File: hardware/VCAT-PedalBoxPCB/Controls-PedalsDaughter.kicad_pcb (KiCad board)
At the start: 2 copper layers, 53 x 58.6 mm, 36 parts, among them J1 MX150_02x03_Vertical, J6 MX150_02x10_Vertical, J7 53307-2471, U3 TLV9301xDCK, U4 TLV70130DBVR, U5 AMC1300BDWV, U6 TLV9301xDCK

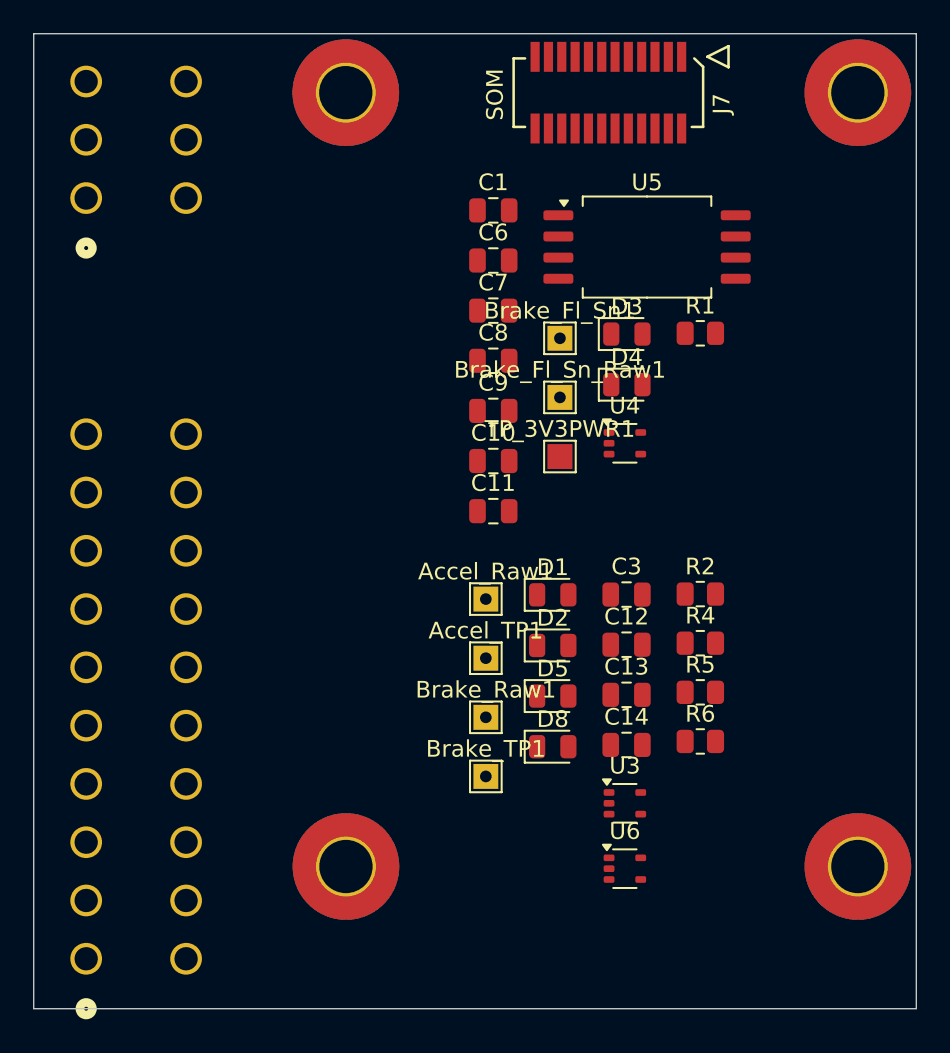
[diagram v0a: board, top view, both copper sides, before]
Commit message: pcb design review #1
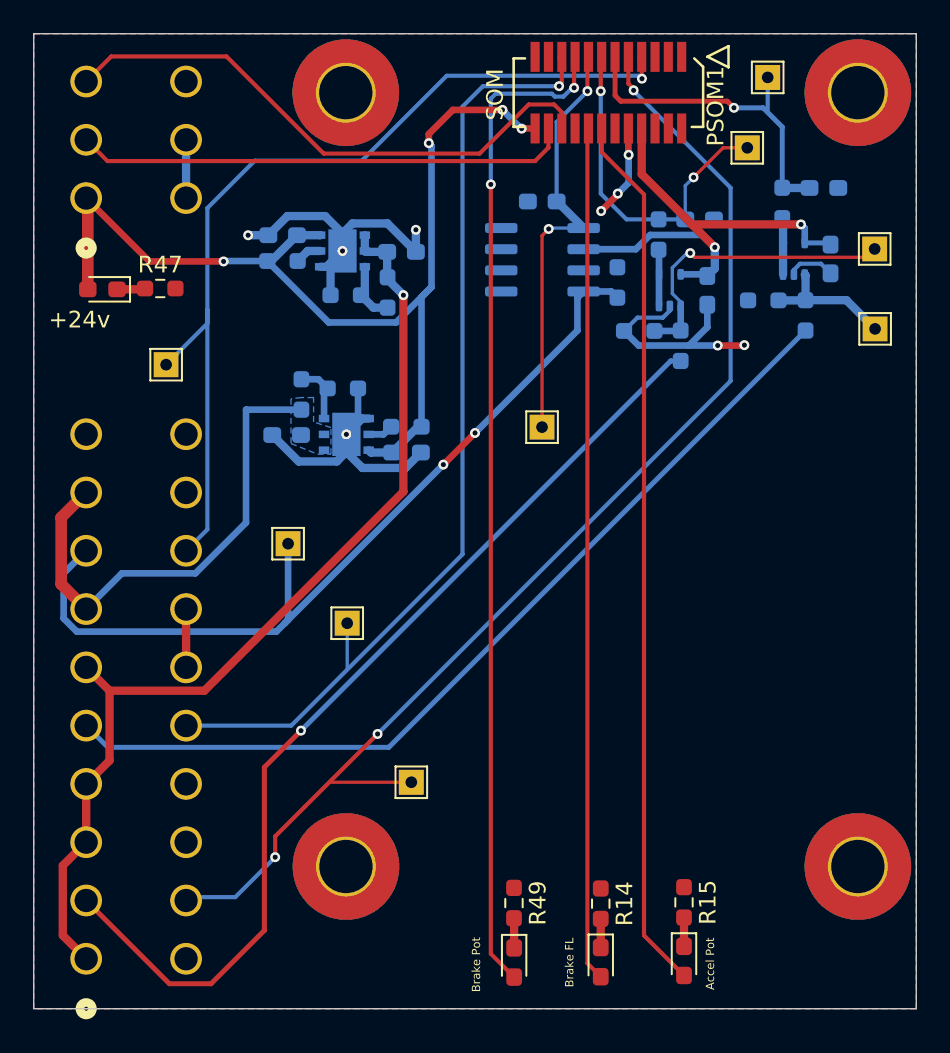
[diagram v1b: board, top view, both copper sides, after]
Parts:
- removed Accel_Raw1: Accel_Raw_TP, TestPoint:TestPoint_THTPad_1.5x1.5mm_Drill0.7mm
- removed Accel_TP1: Accel, TestPoint:TestPoint_THTPad_1.5x1.5mm_Drill0.7mm
- removed Brake_Fl_Sn1: Brake_Fl_Sn_TP, TestPoint:TestPoint_THTPad_1.5x1.5mm_Drill0.7mm
- removed Brake_Fl_Sn_Raw1: Brake_Fl_Sn_Raw_TP, TestPoint:TestPoint_THTPad_1.5x1.5mm_Drill0.7mm
- removed Brake_Raw1: Brake_Raw_TP, TestPoint:TestPoint_THTPad_1.5x1.5mm_Drill0.7mm
- removed Brake_TP1: Brake, TestPoint:TestPoint_THTPad_1.5x1.5mm_Drill0.7mm
- removed C10: 1uF, Capacitor_SMD:C_0805_2012Metric
- removed C11: 100uF, Capacitor_SMD:C_0805_2012Metric
- removed C12, C14: 1nf, Capacitor_SMD:C_0805_2012Metric
- removed C13: 0.1uf, Capacitor_SMD:C_0805_2012Metric
- removed D1, D2, D3, D4, D5, D8: MBR, Diode_SMD:D_0805_2012Metric
- removed TP_3V3PWR1: +3V3PWR, TestPoint:TestPoint_Pad_1.5x1.5mm
- removed U5: AMC1300BDWV, Package_SO:SOIC-8_7.5x5.85mm_P1.27mm
- added +24v: PedalsBoard_Status_Red, LED_SMD:LED_0603_1608Metric_Pad1.05x0.95mm_HandSolder, F.Cu at (125.1, 86.1)
- added Accel Pot: 0603_SMD, LED_SMD:LED_0603_1608Metric_Pad1.05x0.95mm_HandSolder, F.Cu at (160.0, 126.4)
- added AccelPot_Raw: Raw_TP, TestPoint:TestPoint_THTPad_1.5x1.5mm_Drill0.7mm, F.Cu at (171.5, 88.5)
- added AccelPot_Redundant: AccelPotSig, TestPoint:TestPoint_THTPad_1.5x1.5mm_Drill0.7mm, F.Cu at (139.8, 106.2)
- added Accel_GPIO: Accel, TestPoint:TestPoint_THTPad_1.5x1.5mm_Drill0.7mm, F.Cu at (165.0, 73.4)
- added Brake FL: 0603_SMD, LED_SMD:LED_0603_1608Metric_Pad1.05x0.95mm_HandSolder, F.Cu at (155.0, 126.5)
- added Brake Pot: 0603_SMD, LED_SMD:LED_0603_1608Metric_Pad1.05x0.95mm_HandSolder, F.Cu at (149.8, 126.5)
- added BrakeFL_Raw: Brake_Fl_Sn_Raw_TP, TestPoint:TestPoint_THTPad_1.5x1.5mm_Drill0.7mm, F.Cu at (136.2, 101.4)
- added BrakeFl_GPIO: Brake_Fl_Sn_TP, TestPoint:TestPoint_THTPad_1.5x1.5mm_Drill0.7mm, F.Cu at (151.5, 94.4)
- added BrakePot_GPIO: Accel, TestPoint:TestPoint_THTPad_1.5x1.5mm_Drill0.7mm, F.Cu at (163.8, 77.6)
- added BrakePot_Raw: Raw_TP, TestPoint:TestPoint_THTPad_1.5x1.5mm_Drill0.7mm, F.Cu at (171.4, 83.7)
- added BrakePot_Redundant: BrakePotSig, TestPoint:TestPoint_THTPad_1.5x1.5mm_Drill0.7mm, F.Cu at (143.6, 115.7)
- added BrakePress_Redundant: BrakePressSig, TestPoint:TestPoint_THTPad_1.5x1.5mm_Drill0.7mm, F.Cu at (128.9, 90.6)
- added C2: 0.1uf, Capacitor_SMD:C_0603_1608Metric_Pad1.08x0.95mm_HandSolder, B.Cu at (161.4, 86.2)
- added C4: 1uF, Capacitor_SMD:C_0603_1608Metric_Pad1.08x0.95mm_HandSolder, B.Cu at (143.0, 83.8)
- added C5: 1uF, Capacitor_SMD:C_0603_1608Metric_Pad1.08x0.95mm_HandSolder, B.Cu at (135.9, 82.8)
- added R10: 1k, Resistor_SMD:R_0603_1608Metric_Pad0.98x0.95mm_HandSolder, B.Cu at (135.9, 84.4)
- added R11: 100, Resistor_SMD:R_0603_1608Metric_Pad0.98x0.95mm_HandSolder, B.Cu at (165.9, 80.9)
- added R12: 100, Resistor_SMD:R_0603_1608Metric_Pad0.98x0.95mm_HandSolder, B.Cu at (158.5, 82.8)
- added R13: 1k, Resistor_SMD:R_0603_1608Metric_Pad0.98x0.95mm_HandSolder, B.Cu at (143.3, 94.3)
- added R14: 120, Resistor_SMD:R_0603_1608Metric_Pad0.98x0.95mm_HandSolder, F.Cu at (155.0, 123.0)
- added R15: 120, Resistor_SMD:R_0603_1608Metric_Pad0.98x0.95mm_HandSolder, F.Cu at (160.0, 122.9)
- added R3: 10k, Resistor_SMD:R_0603_1608Metric_Pad0.98x0.95mm_HandSolder, B.Cu at (159.8, 89.5)
- added R47: 1.1k, Resistor_SMD:R_0603_1608Metric_Pad0.98x0.95mm_HandSolder, F.Cu at (128.5, 86.0)
- added R49: 120, Resistor_SMD:R_0603_1608Metric_Pad0.98x0.95mm_HandSolder, F.Cu at (149.8, 123.0)
- added R7: 10k, Resistor_SMD:R_0603_1608Metric_Pad0.98x0.95mm_HandSolder, B.Cu at (139.7, 86.5)
- added R8: 1.54k, Resistor_SMD:R_0603_1608Metric_Pad0.98x0.95mm_HandSolder, B.Cu at (137.0, 92.4)
- added R9: 10k, Resistor_SMD:R_0603_1608Metric_Pad0.98x0.95mm_HandSolder, B.Cu at (139.5, 92.0)
- added U1: TLV9301xDCK, Package_TO_SOT_SMD:SOT-353_SC-70-5, B.Cu at (159.2, 86.2)
- added U2: LDO40LPURY, Package_DFN_QFN:DFN-6-1EP_3x3mm_P0.95mm_EP1.7x2.6mm, B.Cu at (139.5, 83.8)
- C1: value 100nF -> 0.01uf; footprint Capacitor_SMD:C_0805_2012Metric -> Capacitor_SMD:C_0603_1608Metric_Pad1.08x0.95mm_HandSolder; moved to B.Cu
- C3, C7, C9: footprint Capacitor_SMD:C_0805_2012Metric -> Capacitor_SMD:C_0603_1608Metric_Pad1.08x0.95mm_HandSolder; moved to B.Cu
- C6: value 100uF -> 0.01uf; footprint Capacitor_SMD:C_0805_2012Metric -> Capacitor_SMD:C_0603_1608Metric_Pad1.08x0.95mm_HandSolder; moved to B.Cu
- C8: value 1nF -> 1uF; footprint Capacitor_SMD:C_0805_2012Metric -> Capacitor_SMD:C_0603_1608Metric_Pad1.08x0.95mm_HandSolder; moved to B.Cu
- R1: value 20 -> 0.175; footprint Resistor_SMD:R_0805_2012Metric -> Resistor_SMD:R_0603_1608Metric_Pad0.98x0.95mm_HandSolder; moved to B.Cu
- R2: value 8.2k -> 10k; footprint Resistor_SMD:R_0805_2012Metric -> Resistor_SMD:R_0603_1608Metric_Pad0.98x0.95mm_HandSolder; moved to B.Cu
- R4: footprint Resistor_SMD:R_0805_2012Metric -> Resistor_SMD:R_0603_1608Metric_Pad0.98x0.95mm_HandSolder; moved to B.Cu
- R5: value 8.2k -> 22k; footprint Resistor_SMD:R_0805_2012Metric -> Resistor_SMD:R_0603_1608Metric_Pad0.98x0.95mm_HandSolder; moved to B.Cu
- R6: value 22k -> 3.16k; footprint Resistor_SMD:R_0805_2012Metric -> Resistor_SMD:R_0603_1608Metric_Pad0.98x0.95mm_HandSolder; moved to B.Cu
- U3: moved to B.Cu
- U4: value TLV70130DBVR -> INA241A5xD; footprint Package_TO_SOT_SMD:SOT-353_SC-70-5 -> Package_SO:SOIC-8_3.9x4.9mm_P1.27mm; moved to B.Cu
- U6: value TLV9301xDCK -> LDO40LPURY; footprint Package_TO_SOT_SMD:SOT-353_SC-70-5 -> Package_DFN_QFN:DFN-6-1EP_3x3mm_P0.95mm_EP1.7x2.6mm; moved to B.Cu
- moved U3 34.2 mm to (166.6, 84.3), turned to 90 degrees
- moved R6 32.9 mm to (142.2, 86.3), turned to -90 degrees
- moved U6 31.0 mm to (139.7, 94.8), turned to 180 degrees
- moved C3 23.6 mm to (168.8, 84.3), turned to 90 degrees
- moved R5 22.0 mm to (157.3, 88.6), turned to 180 degrees
- moved R4 20.9 mm to (164.8, 86.8), turned to 180 degrees
- moved C1 19.9 mm to (168.4, 80.0), turned to 180 degrees
- moved R2 17.9 mm to (167.3, 87.7), turned to -90 degrees
- moved C8 13.2 mm to (136.1, 94.8), turned to 180 degrees
- moved C9 12.9 mm to (151.5, 80.8), turned to 180 degrees
- moved C6 12.6 mm to (160.9, 81.9), turned to 180 degrees
- moved U4 12.1 mm to (151.5, 84.3)
- moved C7 9.99 mm to (143.3, 95.9)
- moved R1 5.84 mm to (156.0, 85.7), turned to 90 degrees
- renumbered J7 to PSOM1
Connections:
- net /Accel renamed Net-(U3--)
- C1 pad 1: +12V -> GNDA
- C1 pad 2: GNDPWR -> /Accel_GPIO
- C3 pad 1: GND -> GNDA
- C3 pad 2: +5V -> +VDDA
- C6 pad 1: +3V3PWR -> GNDA
- C6 pad 2: GNDPWR -> /BrakePot_GPIO
- C7 pad 1: +3V3PWR -> +24V
- C7 pad 2: GNDPWR -> GND
- C8 pad 1: +3V3PWR -> +9V
- C8 pad 2: GNDPWR -> GND
- C9 pad 1: /Brake_Fl -> /BrakeFL_GPIO
- J1 pad 1: unconnected-(J1-+24V-Pad1) -> +24V
- J1 pad 2: unconnected-(J1-CANH_IN-Pad2) -> /CANH_IN
- J1 pad 3: unconnected-(J1-CANL_IN-Pad3) -> /CANL_IN
- J1 pad 4: unconnected-(J1-GND-Pad4) -> GND
- J1 pad 5: unconnected-(J1-CANH_OUT-Pad5) -> GND
- J6 pad 1: unconnected-(J6-+24V-Pad1) -> +5V
- J6 pad 11: unconnected-(J6-GND-Pad11) -> GNDA
- J6 pad 12: unconnected-(J6-CANH_OUT-Pad12) -> /BrakePotRed
- J6 pad 13: unconnected-(J6-CANL_OUT-Pad13) -> GNDA
- J6 pad 14: unconnected-(J6-GND_OUT*-Pad14) -> GNDA
- J6 pad 15: unconnected-(J6-Pad15) -> /AccelPotRed
- J6 pad 16: unconnected-(J6-Pad16) -> GNDA
- J6 pad 17: unconnected-(J6-Pad17) -> GNDA
- J6 pad 18: unconnected-(J6-Pad18) -> /BrakePressRed
- J6 pad 19: unconnected-(J6-Pad19) -> GNDA
- J6 pad 2: unconnected-(J6-CANH_IN-Pad2) -> /BrakePot_ADC
- J6 pad 3: unconnected-(J6-CANL_IN-Pad3) -> +5V
- J6 pad 4: unconnected-(J6-PWR_OUT*-Pad4) -> +5V
- J6 pad 5: unconnected-(J6-Pad5) -> /Accel_ADC
- J6 pad 6: unconnected-(J6-Pad6) -> +5V
- J6 pad 7: unconnected-(J6-Pad7) -> +9V
- J6 pad 8: unconnected-(J6-Pad8) -> /BrakeFL_ADC
- J6 pad 9: unconnected-(J6-Pad9) -> +9V
- PSOM1 pad 1: unconnected-(J7-GND-Pad1) -> GND
- PSOM1 pad 10: unconnected-(J7-GNDA-Pad10) -> GNDA
- PSOM1 pad 11: unconnected-(J7-ADC1_IN9-Pad11) -> /Accel_GPIO
- PSOM1 pad 13: unconnected-(J7-ADC1_IN10-Pad13) -> /BrakePot_GPIO
- PSOM1 pad 14: unconnected-(J7-SPI2_MISO-Pad14) -> /AccelPotStatus
- PSOM1 pad 15: unconnected-(J7-ADC1_IN11-Pad15) -> /BrakeFL_GPIO
- PSOM1 pad 16: unconnected-(J7-SPI2_MOSI-Pad16) -> /BrakeFluidStatus
- PSOM1 pad 17: unconnected-(J7-SPI1_MOSI-Pad17) -> /BrakePotStatus
- PSOM1 pad 19: unconnected-(J7-SPI1_NSS-Pad19) -> /AccelPotRed
- PSOM1 pad 2: unconnected-(J7-+3.3v-Pad2) -> +3.3V
- PSOM1 pad 20: unconnected-(J7-CAN_L-Pad20) -> /CANL_IN
- PSOM1 pad 22: unconnected-(J7-CAN_H-Pad22) -> /CANH_IN
- PSOM1 pad 24: unconnected-(J7-+24V_In-Pad24) -> +24V
- PSOM1 pad 3: unconnected-(J7-GND-Pad3) -> GND
- PSOM1 pad 5: unconnected-(J7-GND-Pad5) -> GND
- PSOM1 pad 7: unconnected-(J7-OPAMP1_VINP-Pad7) -> /BrakePressRed
- PSOM1 pad 8: unconnected-(J7-VDDA-Pad8) -> +VDDA
- PSOM1 pad 9: unconnected-(J7-ADC1_IN7-Pad9) -> /BrakePotRed
- R1 pad 1: /Brake Fluid Sensor/INP -> /BrakeFL_ADC
- R1 pad 2: GNDPWR -> GNDA
- R2 pad 2: unconnected-(R2-Pad2) -> /Accel_ADC
- R4 pad 2: GND -> GNDA
- R5 pad 1: Net-(U6-+) -> Net-(U1-+)
- R5 pad 2: unconnected-(R5-Pad2) -> GNDA
- R6 pad 1: Net-(U6-+) -> +5V
- R6 pad 2: GND -> Net-(U2-ADJ)
- U3 pad 2: GND -> GNDA
- U3 pad 5: +5V -> +VDDA
- U4 pad 1: +12V -> GNDA
- U4 pad 2: unconnected-(U4-NC-Pad2) -> GNDA
- U4 pad 3: unconnected-(U4-NC-Pad3) -> GNDA
- U4 pad 4: GNDPWR -> GNDA
- U4 pad 5: +3V3PWR -> /BrakeFL_GPIO
- U6 pad 1: Net-(U6-+) -> GND
- U6 pad 2: GND -> Net-(U6-EN)
- U6 pad 3: /Brake_Pot -> +24V
- U6 pad 4: /Brake_Pot -> +9V
- U6 pad 5: +5V -> +9V
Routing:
- net /BrakePotRed: track 0.00 -> 75.4 mm, vias 0 -> 3
- net +24V: track 0.00 -> 63.5 mm, vias 0 -> 4
- net /AccelPotRed: track 0.00 -> 63.4 mm, vias 0 -> 1
- net /BrakePotStatus: track 0.00 -> 60.6 mm, vias 0 -> 2
- net +5V: track 0.00 -> 59.5 mm, vias 0 -> 1
- net /BrakePot_ADC: track 0.00 -> 59.0 mm, vias 0 -> 1
- net /BrakePressRed: track 0.00 -> 56.2 mm, vias 0 -> 1
- net /Accel_ADC: track 0.00 -> 54.1 mm
- net /AccelPotStatus: track 0.00 -> 52.9 mm
- net /BrakeFL_ADC: track 0.00 -> 52.8 mm, vias 0 -> 2
- net /BrakeFluidStatus: track 0.00 -> 51.3 mm
- net GND: track 0.00 -> 38.9 mm, vias 0 -> 4
- net /CANL_IN: track 0.00 -> 34.0 mm
- net +VDDA: track 0.00 -> 30.4 mm, vias 0 -> 2
- net +9V: track 0.00 -> 30.1 mm
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- added copper zone on B.Cu, net +9V
- added copper zone on F.Cu, net GND
- added copper zone on B.Cu, net GNDA
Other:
- board text added: "Adj LDO 5V"
- board text added: "Adj LDO 9V"
